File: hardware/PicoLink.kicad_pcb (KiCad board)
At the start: 2 copper layers, 50 parts, among them J2 USB_C_Receptacle_USB2.0_14P, J3 ARM_JTAG_10Pin, J4 TARGET, J7 UART, J8 SIGROK_INPUT, J9 SIGROK_ADC, SW2 BOOT SELECTOR, U4 W25Q16JVSS, U6 AMS1117-3.3, Y2 12Mhz HC49-SD

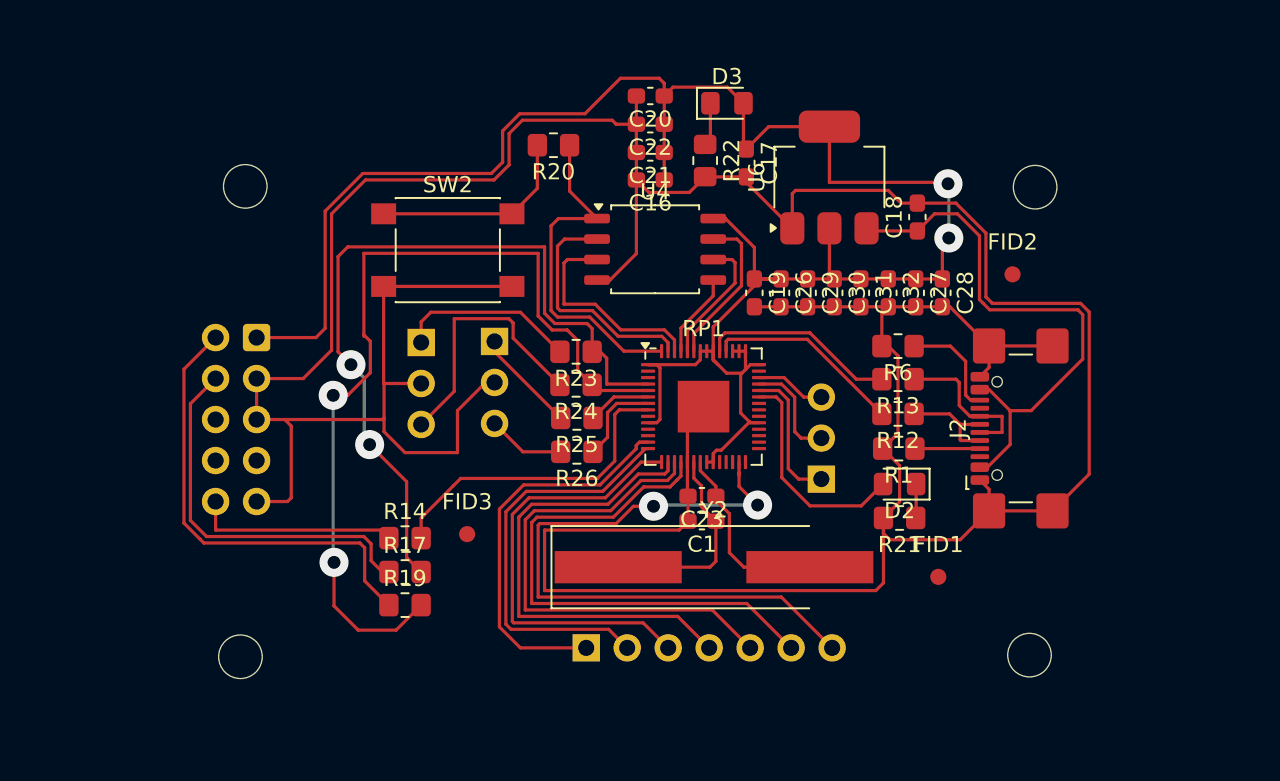
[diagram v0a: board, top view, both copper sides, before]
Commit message: [07-17-1304] add edge cut
Update README.md
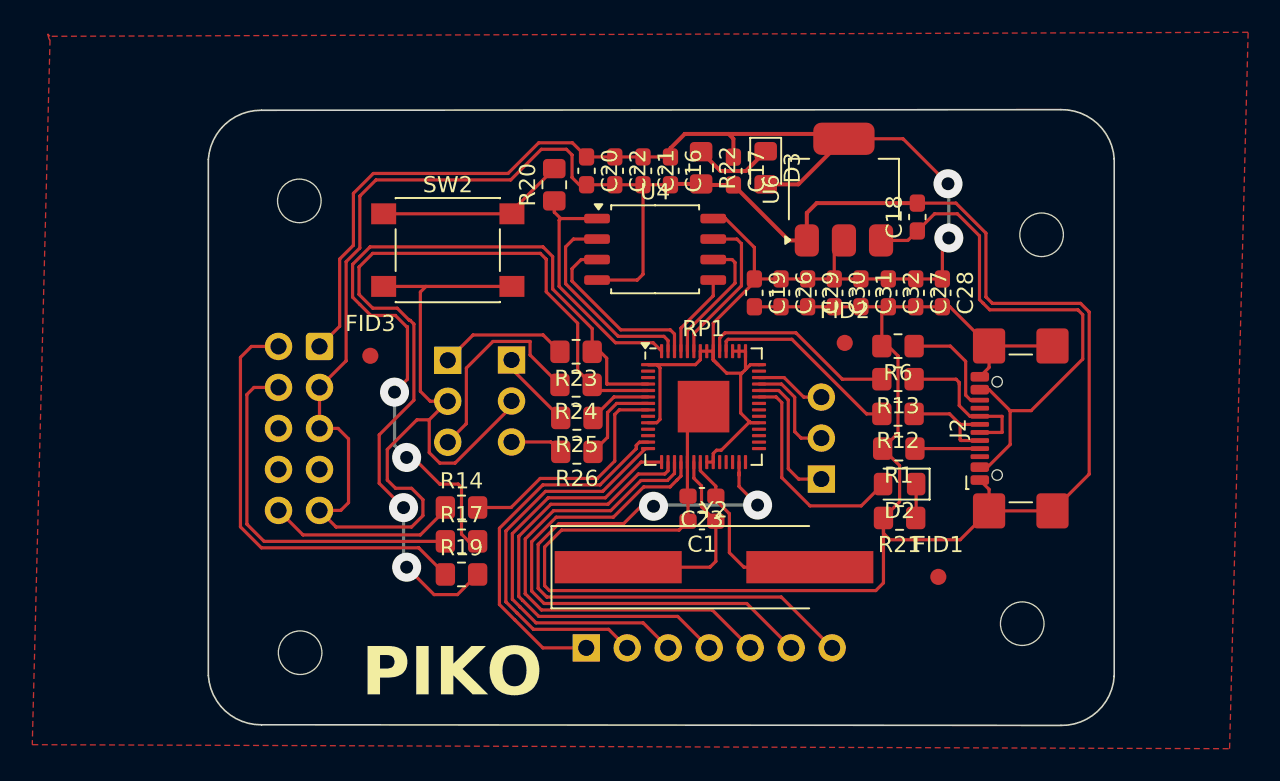
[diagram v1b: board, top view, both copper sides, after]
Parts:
- J8: footprint Connector_PinHeader_2.54mm:PinHeader_1x07_P2.54mm_Horizontal -> Connector_PinHeader_2.54mm:PinHeader_1x07_P2.54mm_Vertical
- moved FID3 12.6 mm to (135.1, 89.5)
- moved FID2 11.2 mm to (164.4, 88.7)
- moved C20 6.09 mm to (148.5, 78.0), turned to -90 degrees
- moved D3 4.66 mm to (159.6, 77.8), turned to -90 degrees
- moved R17 3.98 mm to (140.7, 101.0)
- moved R19 3.98 mm to (140.7, 103.0)
- moved R14 3.98 mm to (140.7, 98.9)
- moved J3 3.94 mm to (131.9, 88.9)
- moved H4 3.71 mm to (130.7, 107.9)
- moved C22 3.63 mm to (150.2, 78.0), turned to -90 degrees
- moved H6 3.47 mm to (130.7, 79.9)
- moved H5 2.98 mm to (176.7, 82.0)
- moved R20 2.45 mm to (146.4, 78.9), turned to 90 degrees
- moved H3 2.00 mm to (175.4, 106.1)
- moved J4 1.98 mm to (139.8, 89.8)
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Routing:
- net +3.3V: track 126.1 -> 115.5 mm
- net /SPI_SS_N: track 21.4 -> 15.8 mm
- net TGT_RESET: track 19.8 -> 14.8 mm
- net GND: track 245.7 -> 242.1 mm
- net Net-(J4-Pin_1): track 11.1 -> 8.03 mm
- net Net-(J4-Pin_3): track 16.2 -> 13.2 mm
- net Net-(D3-K): track 2.68 -> 5.00 mm
- net TGT_SWDIO: track 54.8 -> 52.8 mm
- net /SPI_SD1: track 14.7 -> 12.9 mm
- net /SPI_SD2: track 13.2 -> 11.3 mm
- net Net-(J7-Pin_1): track 6.44 -> 4.85 mm
- net Net-(J7-Pin_3): track 4.83 -> 3.30 mm
- net /SIGROK_IN2: track 25.5 -> 24.0 mm
- net /SIGROK_IN3: track 27.6 -> 26.1 mm
- net /SIGROK_IN1: track 24.3 -> 22.8 mm
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- added copper zone on F.Cu, net +3.3V
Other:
- board outline added: 56.1 x 38.2 mm
- board text added: "PIKO"
